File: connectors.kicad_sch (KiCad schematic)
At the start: 4 parts, among them J1 Conn_02x03_Odd_Even, J2 Conn_01x09_Pin, J3 Conn_01x04_Pin, J4 Conn_01x04_Pin

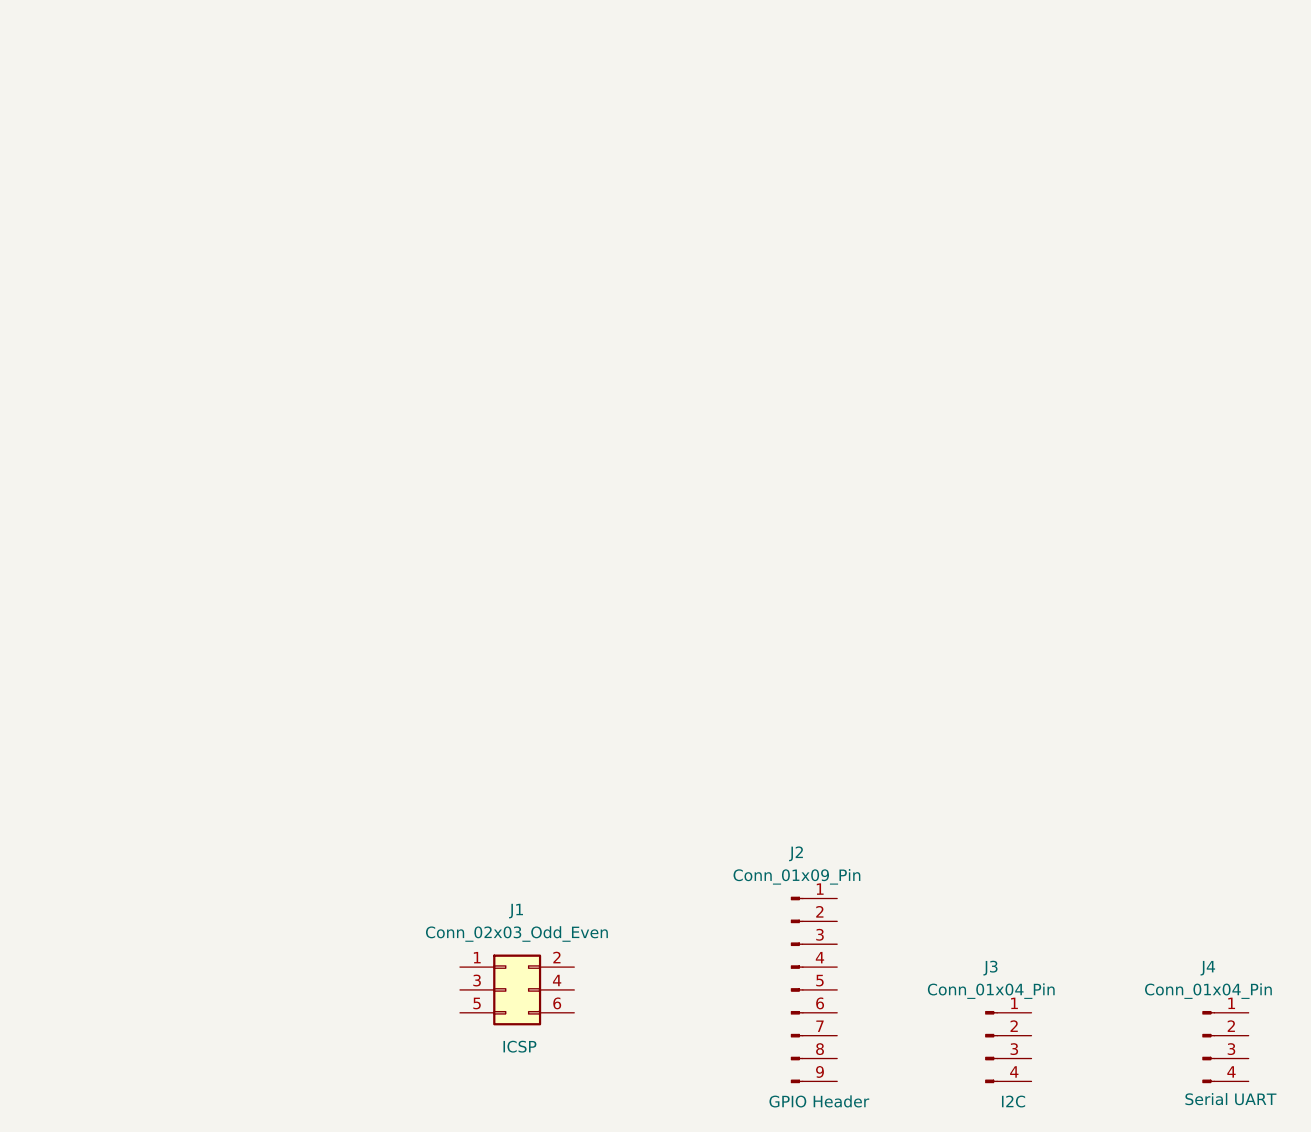
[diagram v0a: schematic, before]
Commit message: completed comments
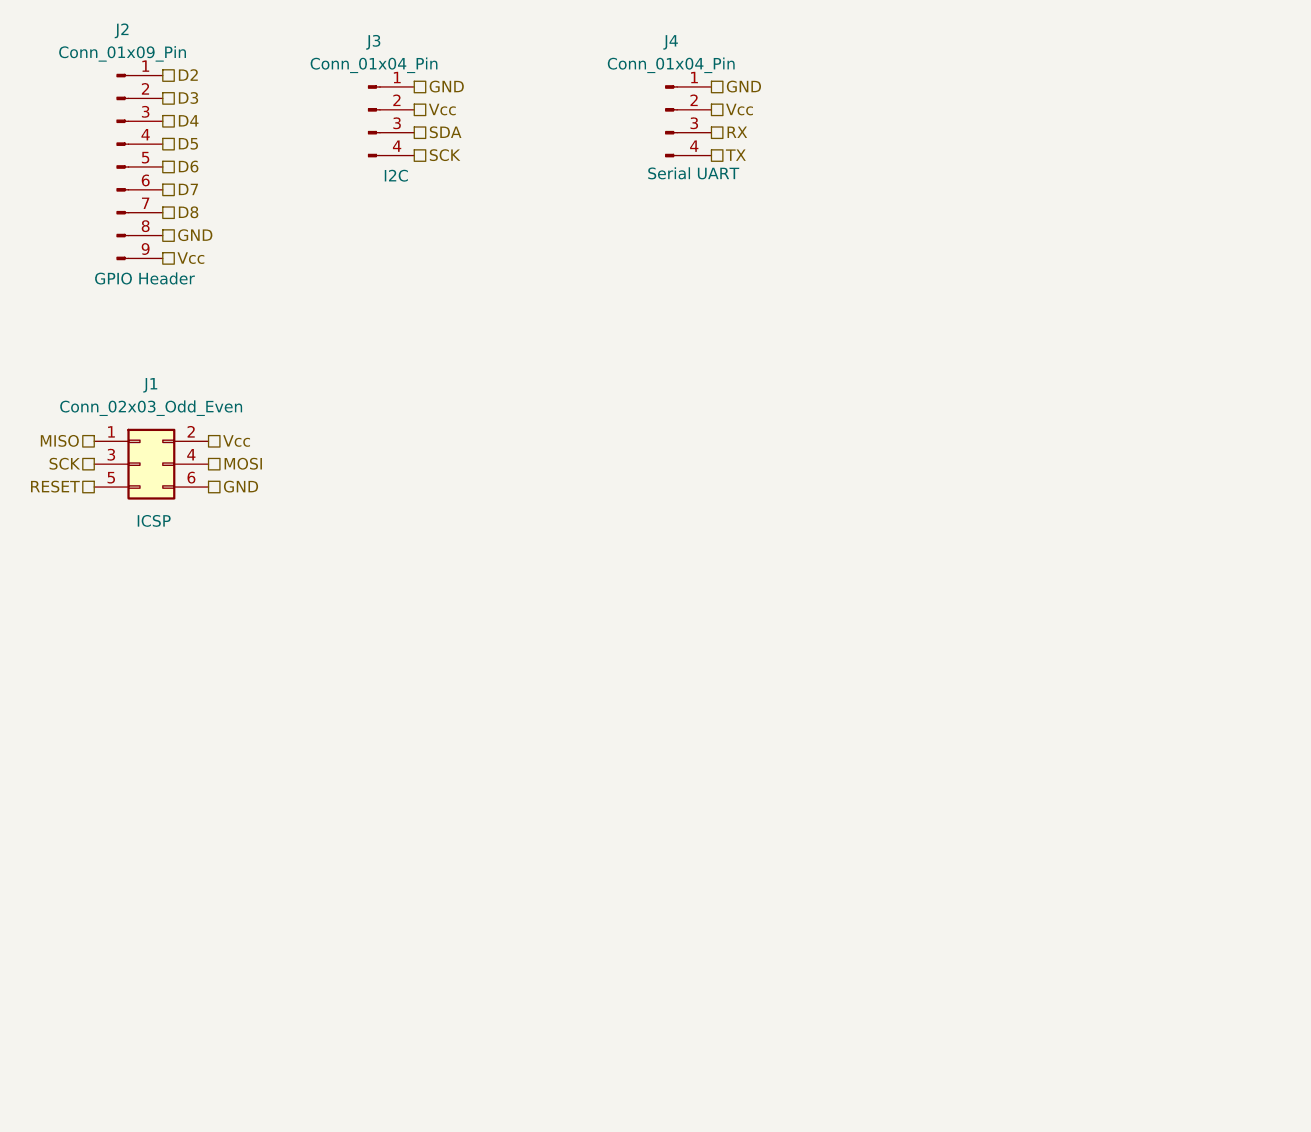
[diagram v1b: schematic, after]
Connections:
- net MISO: now reaches J1.1 (Pin_1)
- net Vcc: now reaches J1.2 (Pin_2)
- net Vcc: now also J2.9 (Pin_9), J3.2 (Pin_2), J4.2 (Pin_2)
- net SCK: now reaches J1.3 (Pin_3)
- net SCK: now also J3.4 (Pin_4)
- net MOSI: now reaches J1.4 (Pin_4)
- net RESET: now reaches J1.5 (Pin_5)
- net GND: now reaches J1.6 (Pin_6)
- net GND: now also J2.8 (Pin_8), J3.1 (Pin_1), J4.1 (Pin_1)
- net SDA: now reaches J3.3 (Pin_3)
- net RX: now reaches J4.3 (Pin_3)
- net TX: now reaches J4.4 (Pin_4)
- net D2: now reaches J2.1 (Pin_1)
- net D3: now reaches J2.2 (Pin_2)
- net D4: now reaches J2.3 (Pin_3)
- net D5: now reaches J2.4 (Pin_4)
- net D6: now reaches J2.5 (Pin_5)
- net D7: now reaches J2.6 (Pin_6)
- net D8: now reaches J2.7 (Pin_7)
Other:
- moved on the sheet: J1, J2, J3, J4
